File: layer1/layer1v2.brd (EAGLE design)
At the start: 17.8 x 48.3 mm, 15 parts, among them U1 microSD, U2 DS3234, U3 MMA8452Q

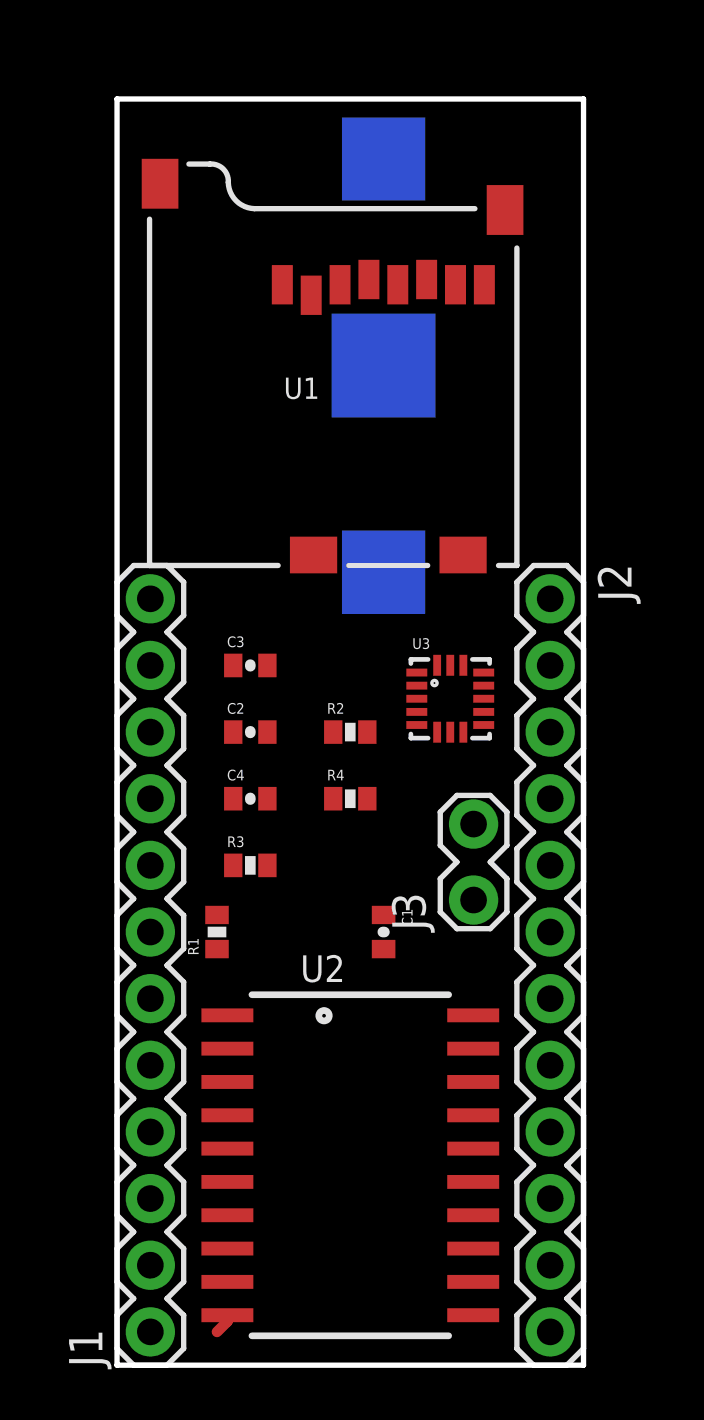
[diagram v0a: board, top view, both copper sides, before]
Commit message: ops
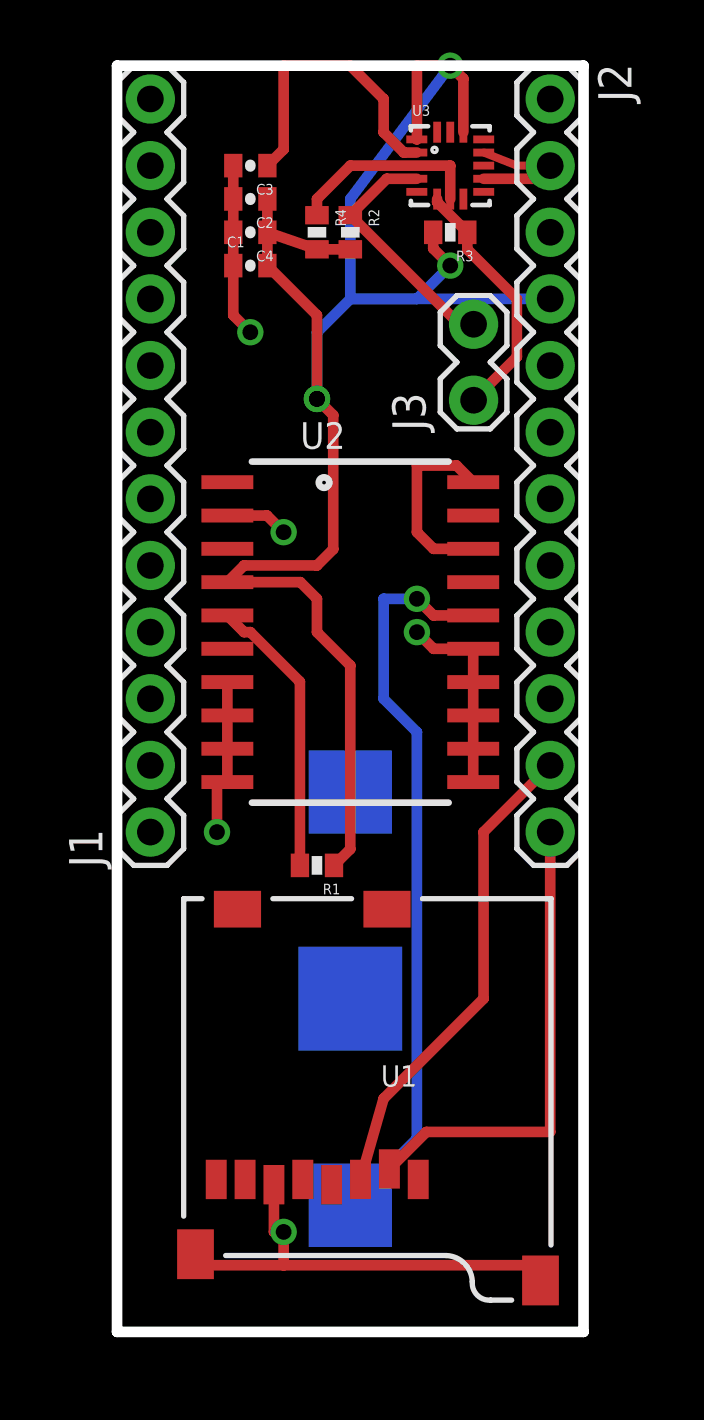
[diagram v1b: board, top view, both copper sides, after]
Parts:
- moved C1 25.9 mm to (5.08, 41.9), turned to 0 degrees
- moved R3 25.3 mm to (12.7, 43.2), turned to 180 degrees
- moved BAT1 24.2 mm to (8.89, 14.0)
- moved R4 21.6 mm to (7.62, 43.2), turned to 270 degrees
- moved C4 21.6 mm to (5.08, 43.2), turned to 180 degrees
- moved C2 20.3 mm to (5.08, 44.5), turned to 180 degrees
- moved U2 20.3 mm to (8.89, 27.9)
- moved U3 20.3 mm to (12.7, 45.7)
- moved J1 19.1 mm to (1.27, 20.3)
- moved J3 19.1 mm to (13.6, 37.0)
- moved R2 19.1 mm to (8.89, 43.2), turned to 270 degrees
- moved C3 19.0 mm to (5.08, 45.7), turned to 180 degrees
- moved J2 19.0 mm to (16.5, 48.3)
- moved U1 18.0 mm to (2.54, 17.8), turned to 180 degrees
- moved R1 4.58 mm to (7.62, 19.1), turned to 180 degrees
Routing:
- net VCC: track 0.00 -> 67.4 mm, vias 0 -> 3
- net GND: track 0.80 -> 45.9 mm, vias 0 -> 5
- net VBATT: track 0.00 -> 28.4 mm, vias 0 -> 1
- net MOSI: track 0.00 -> 18.5 mm
- net SD_CS: track 0.00 -> 18.1 mm
- net BYP: track 0.00 -> 11.3 mm
- net INT/SQW: track 0.00 -> 10.8 mm
- net SDA: track 0.00 -> 9.61 mm
- net SCL: track 0.00 -> 9.53 mm
- net SA0: track 0.00 -> 7.50 mm
- net SCK: track 0.00 -> 7.36 mm
- net N$1: track 0.00 -> 4.34 mm
- removed copper zone on layer 16, net GND
